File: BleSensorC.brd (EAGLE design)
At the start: 29.5 x 37.5 mm, 14 parts, among them IC1 SI7020-A10-GM, U1 PIC18(L)F14K22-SOIC

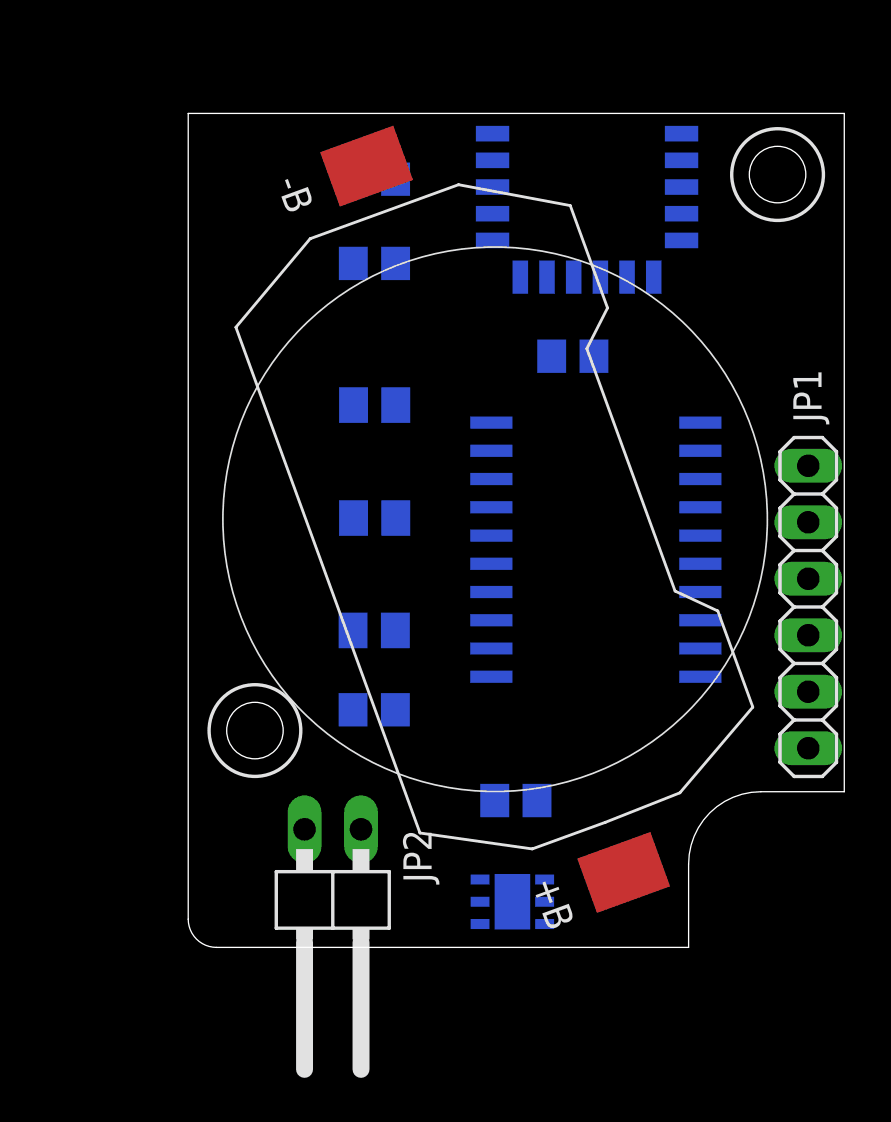
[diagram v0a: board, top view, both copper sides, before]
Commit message: Fusion 3D support
Fusion 3D support
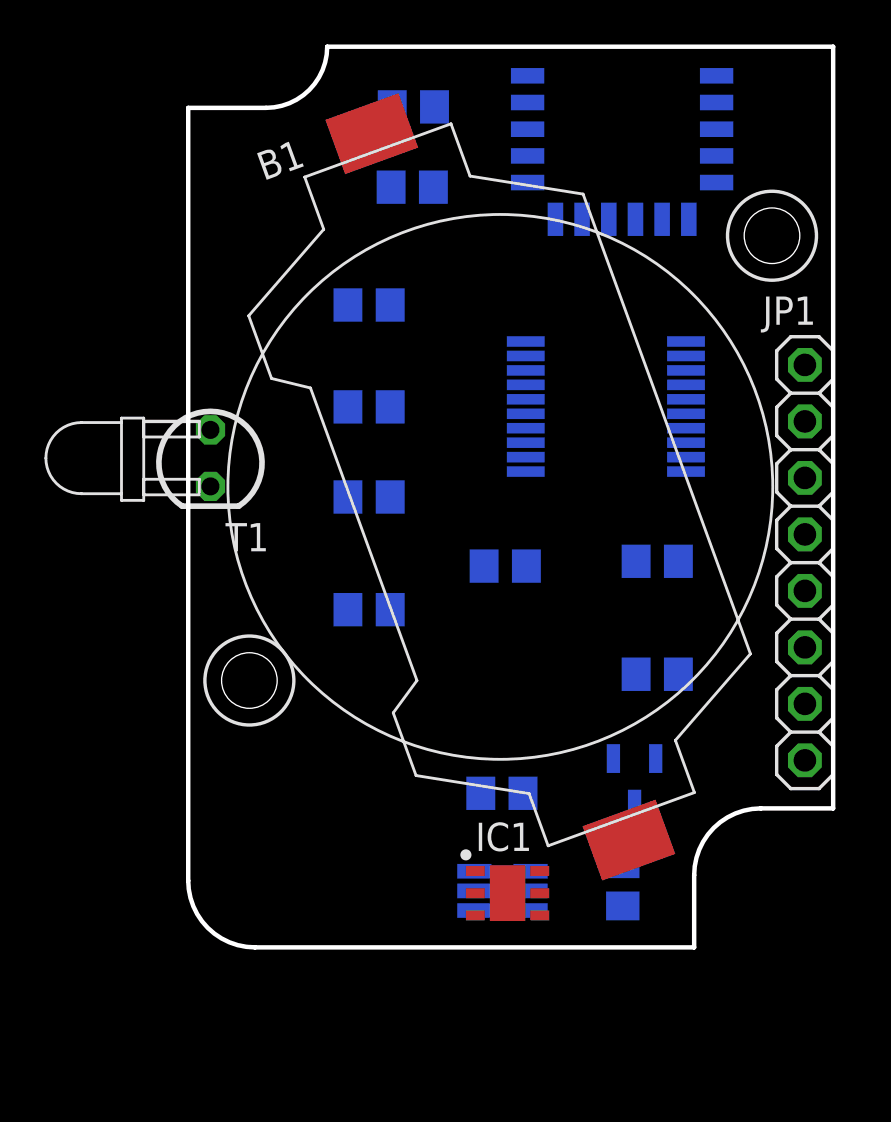
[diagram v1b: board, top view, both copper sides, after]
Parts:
- removed JP2: (no value), pinhead:1X02/90
- removed U$3: SMTU2450N-LF, Battery holders:SMD2450
- added B1: SMTU2450N-LF.TR, esao:SMTU2450N-LF
- added C6: 1nF, resistor:C0805
- added C7: 1uF, resistor:C0805
- added MK1: SPH0644HM4H-1-3D, esao:SOJ88P324X95-6
- added Q1: SI2333DDS-T1-GE3, esao:SOT95P237X112-3
- added R4: 4k7, resistor:R0805
- added T1: BPW85C-L90, esao:LED-3MM
- C5: value 1nF -> 100nF
- IC1: value SI7020-A10-GM -> SI7020-A20-GM; device si70xx-10:DFN6-3X3 -> esao:SON100P300X300X80-7N
- JP1: value (none) -> PINHD-1X8; device pinhead:1X06 -> esao:1X08-S
- R1, R2, R3: device resistor:M0805 -> resistor:R0805
- U1: value PIC18(L)F14K22-SOIC -> PIC16LF18446-I_SS; device Microchip PIC18F12K44_esao:SOIC-20 -> SamacSys_Parts:SOP65P780X200-20
- U2: value (none) -> RN4871-I; device Microchip RN4871:RN4871 -> esao:RN4871
- moved C5 13.7 mm to (19.5, 2.81), turned to 90 degrees
- moved C3 9.97 mm to (21.1, 17.4)
- moved R1 6.00 mm to (8.13, 20.3)
- moved U1 5.86 mm to (18.8, 24.3), turned to 180 degrees
- moved R2 5.01 mm to (8.13, 24.3)
- moved R3 4.51 mm to (8.13, 28.9)
- moved C1 3.83 mm to (10.1, 34.2)
- moved C2 3.69 mm to (10.1, 37.8)
- moved U2 3.58 mm to (20.0, 37.0)
- moved JP1 2.29 mm to (29.0, 17.3)
- moved C4 0.71 mm to (14.1, 6.93), turned to 180 degrees
- moved IC1 0.44 mm to (14.4, 2.44), flipped to the top
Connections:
- net RA3_MCLR_VPP renamed !MCLR!_VPP_RA3
- removed net SCL: IC1.6, R3.2, U1.11
- removed net SDA: IC1.1, R2.2, U1.13
- removed net U_MON: U1.17
- new net +B: B1.+B, Q1.3
- new net SCL1: IC1.6, R3.2, U1.16
- new net SCL2: MK1.2, U1.8
- new net SDA1: IC1.1, R2.2, U1.15
- new net SDA2: MK1.3, U1.9
- net GND: now also B1.-B, C6.2, C7.2, IC1.7, MK1.4, MK1.6, Q1.1; no longer U$3.B-
- net IMP: now also C6.1, T1.K; no longer C5.1, JP2.2
- net PIC_RX: now also U1.5; no longer U1.12
- net PIC_TX: now also U1.6; no longer U1.10
- net RST: now also C7.1, R4.1
- net UART_RX_IND: now also U1.7; no longer U1.16
- net VDD: now also C5.1, MK1.1, MK1.5, Q1.2, R4.2, T1.A; no longer JP2.1, U$3.B+
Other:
- board size 29.5 x 37.5 mm -> 29 x 40.5 mm
